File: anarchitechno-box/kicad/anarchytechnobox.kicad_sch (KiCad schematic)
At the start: 18 parts, among them J3 Screw_Terminal_01x02, J4 Screw_Terminal_01x02, J5 Screw_Terminal_01x02, J6 Screw_Terminal_01x02, U1 TME-0503S, U2 L7805, U3 LM7812_TO220

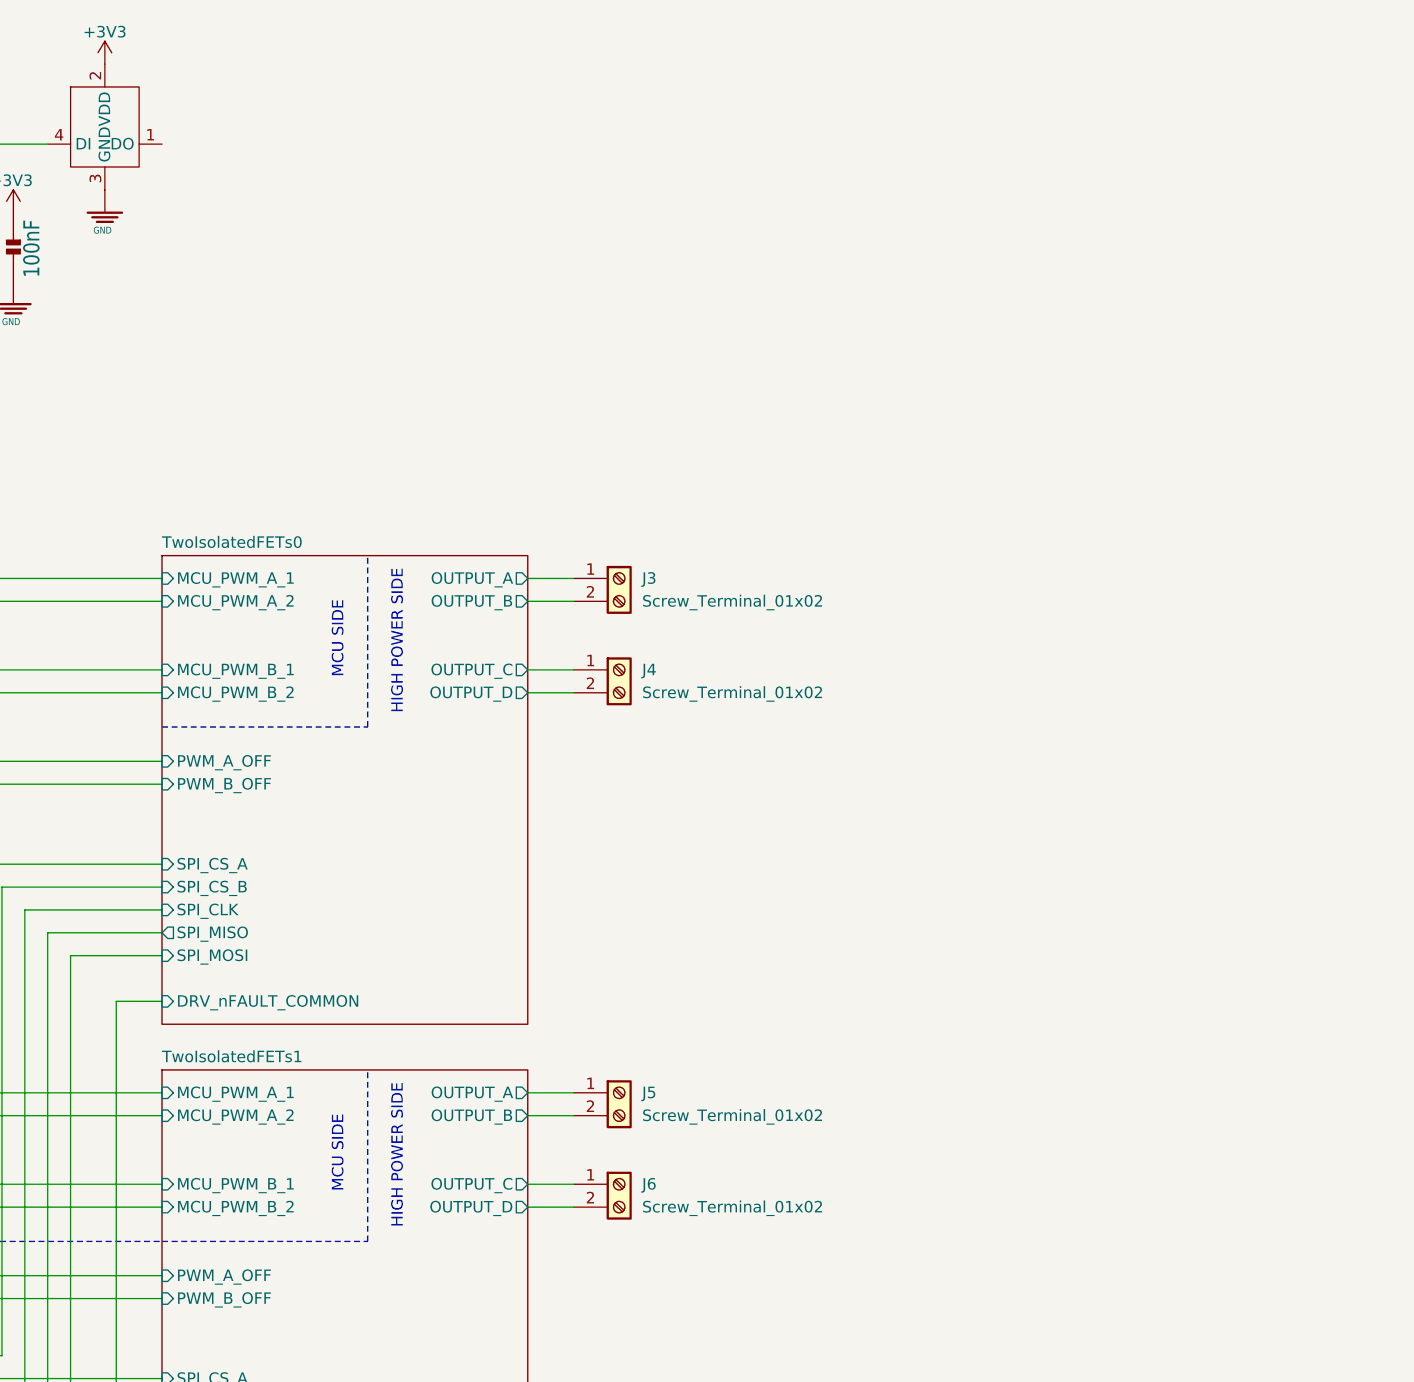
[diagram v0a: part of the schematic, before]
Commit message: meer Stijn in de Trein
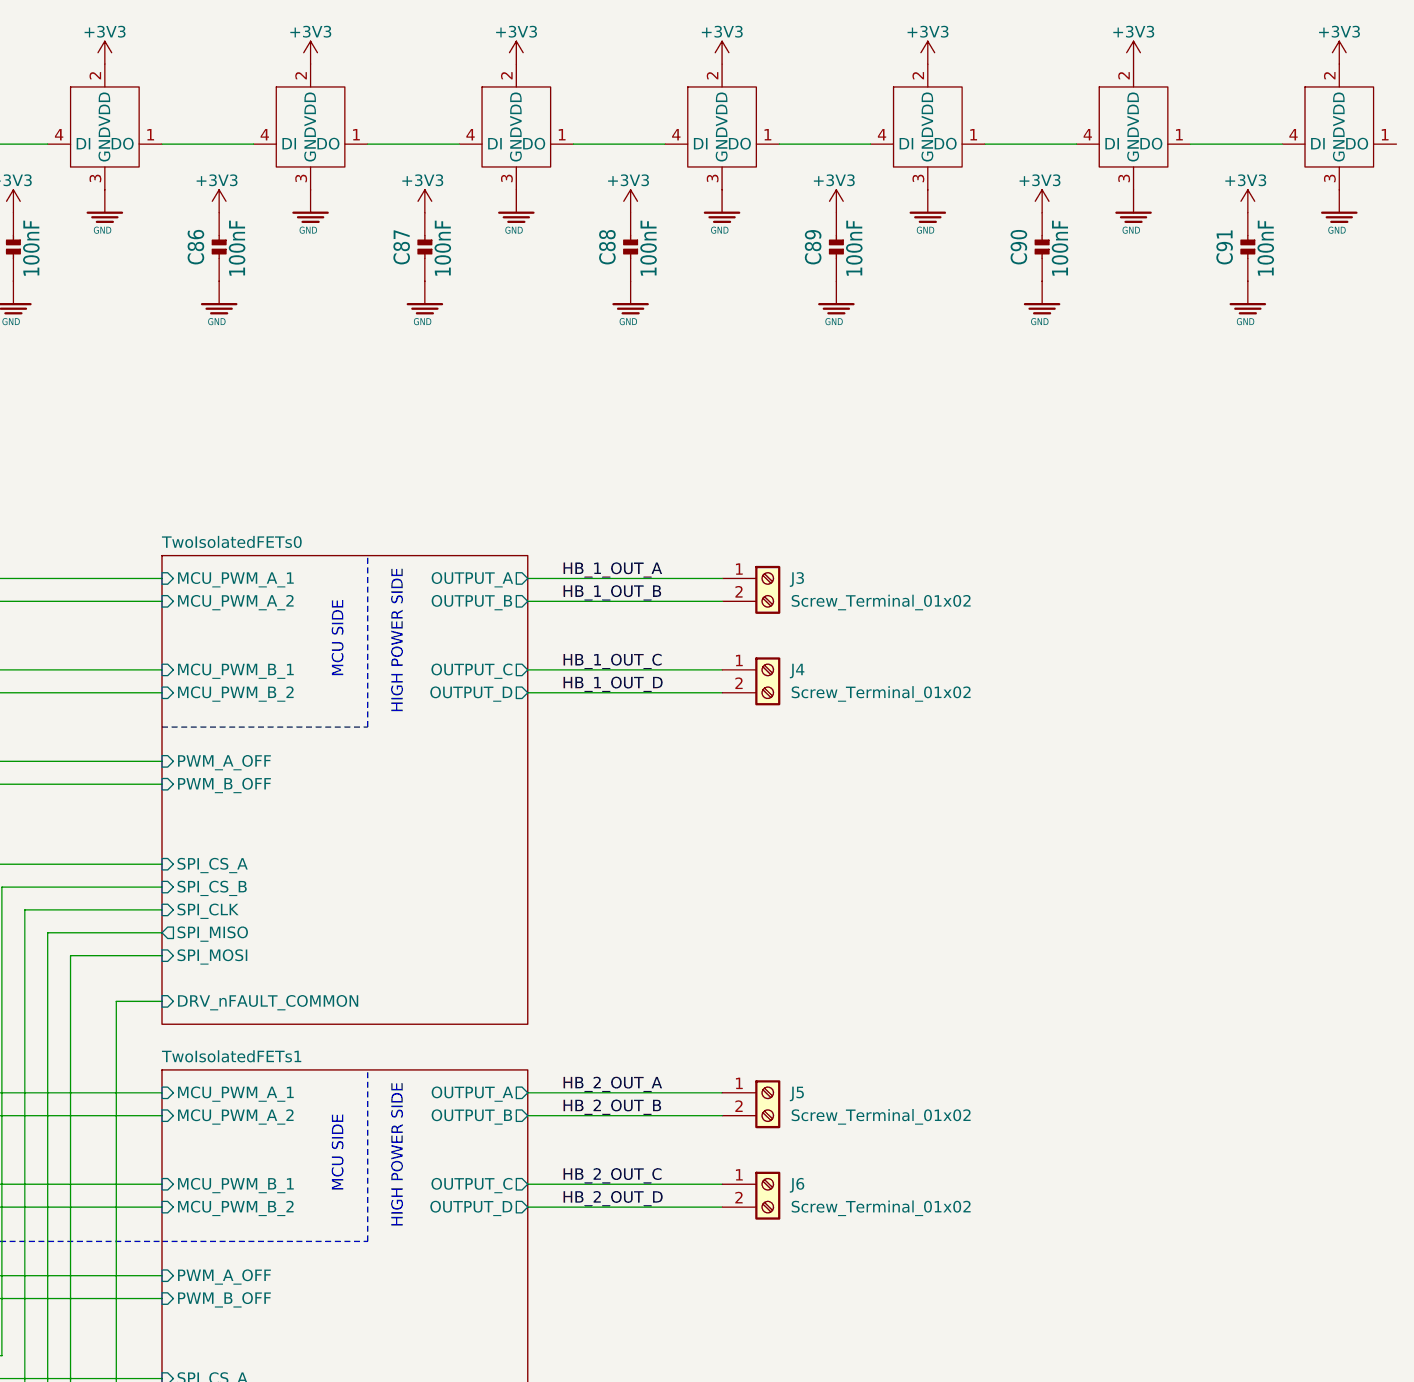
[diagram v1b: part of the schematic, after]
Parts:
- added C86, C87, C88, C89, C90, C91: 100nF, Capacitor_SMD:C_0402_1005Metric, symbol TINRS - Wobbler (pico)sch-eagle-import:C-EUC0402
- added D18, D19, D20, D21, D22, D23: C5349953, TinyLEDs:XL-1010, symbol TinyLEDs:XL-1010
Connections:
- net +3V3: now also C86.2, C87.2, C88.2, C89.2, C90.2, C91.2, D18.2 (VDD), D19.2 (VDD), D20.2 (VDD), D21.2 (VDD), D22.2 (VDD), D23.2 (VDD)
- net GND: now also C86.1, C87.1, C88.1, C89.1, C90.1, C91.1, D18.3 (GND), D19.3 (GND), D20.3 (GND), D21.3 (GND), D22.3 (GND), D23.3 (GND)
- net at D3.1 (DO): now also D18.4 (DI)
- net TwoIsolatedFETs0/OUTPUT_A renamed HB_1_OUT_A
- net TwoIsolatedFETs0/OUTPUT_B renamed HB_1_OUT_B
- net TwoIsolatedFETs0/OUTPUT_C renamed HB_1_OUT_C
- net TwoIsolatedFETs0/OUTPUT_D renamed HB_1_OUT_D
- net TwoIsolatedFETs1/OUTPUT_A renamed HB_2_OUT_A
- net TwoIsolatedFETs1/OUTPUT_B renamed HB_2_OUT_B
- net TwoIsolatedFETs1/OUTPUT_C renamed HB_2_OUT_C
- net TwoIsolatedFETs1/OUTPUT_D renamed HB_2_OUT_D
- new net: D22.1 (DO), D23.4 (DI)
- new net: D21.1 (DO), D22.4 (DI)
- new net: D20.1 (DO), D21.4 (DI)
- new net: D18.1 (DO), D19.4 (DI)
- new net: D19.1 (DO), D20.4 (DI)
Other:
- moved on the sheet: J3, J4, J5, J6
